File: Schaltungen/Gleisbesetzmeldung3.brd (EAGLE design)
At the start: 81 parts, among them IC1 CNY-17-2, IC10 S462, IC11 CNY-17-2, IC12 S462, IC13 CNY-17-2, IC14 S462, IC15 CNY-17-2, IC16 S462, IC2 S462, IC3 CNY-17-2, IC4 S462, IC5 CNY-17-2, IC6 S462, IC7 CNY-17-2, IC8 S462, IC9 CNY-17-2

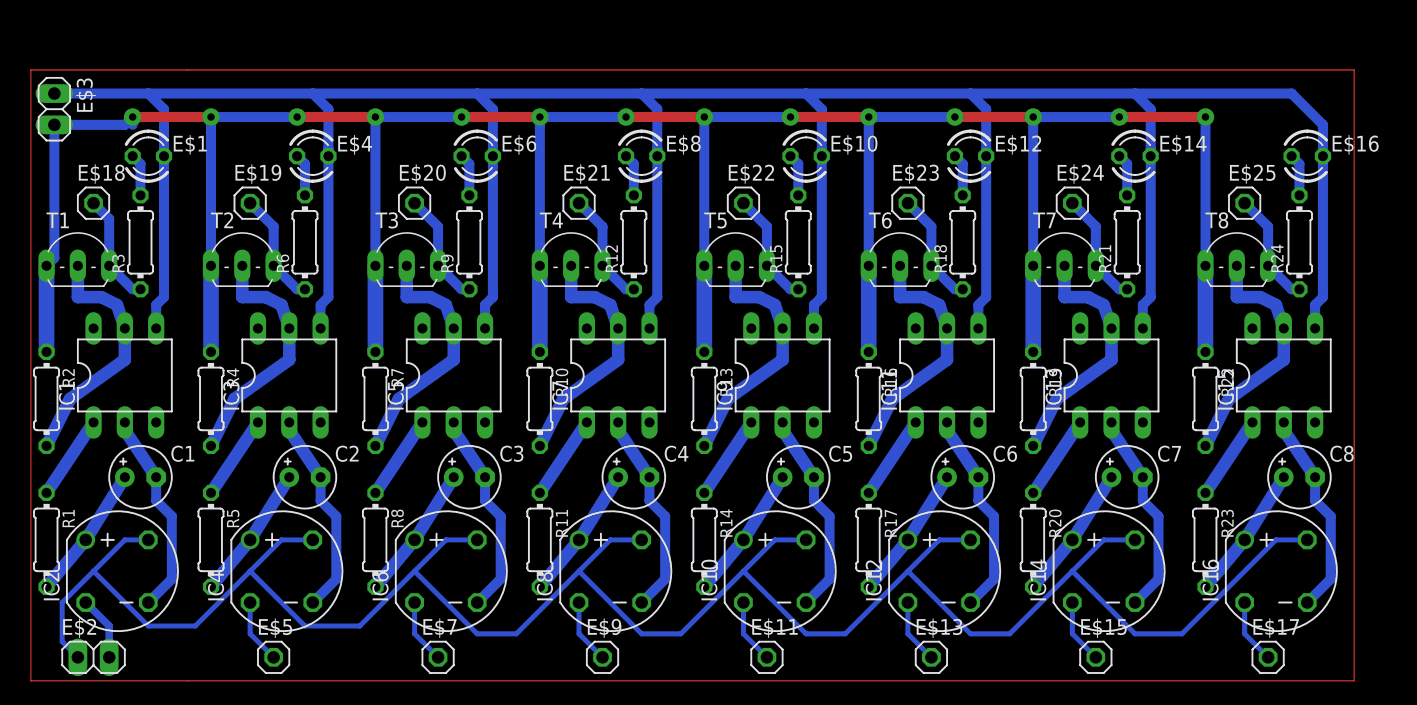
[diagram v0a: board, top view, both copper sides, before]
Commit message: update
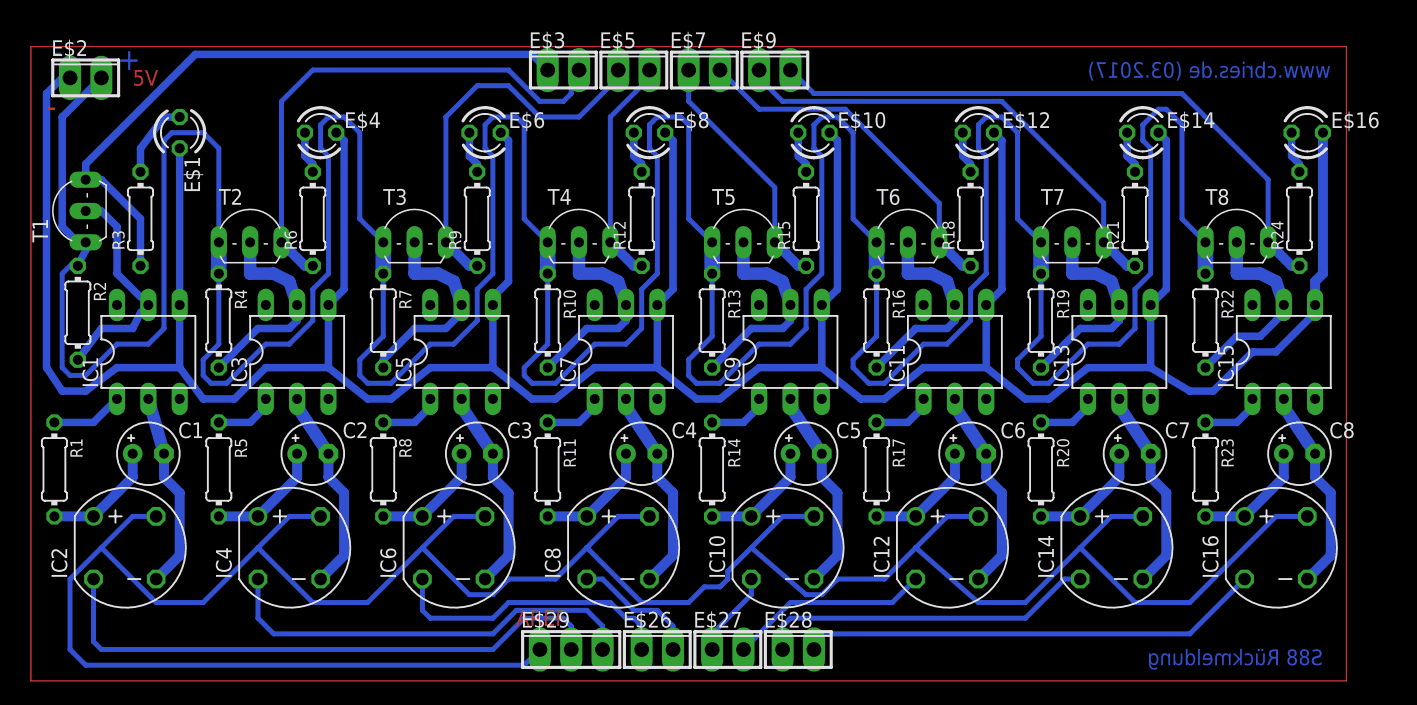
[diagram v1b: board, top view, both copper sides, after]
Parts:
- removed E$11, E$13, E$15, E$17, E$18, E$19, E$20, E$21, E$22, E$23, E$24, E$25: (no value), pinhead:1X01
- added E$26, E$27, E$28: (no value), con-phoenix-254:2POL254
- added E$29: (no value), con-phoenix-254:3POL254
- E$2, E$3: device pinhead:1X02 -> con-phoenix-254:2POL254
- E$5, E$7, E$9: device pinhead:1X01 -> con-phoenix-254:2POL254
- moved E$5 55.9 mm to (48.9, 49.5)
- moved E$7 52.3 mm to (54.6, 49.5)
- moved E$9 49.6 mm to (60.3, 49.5)
- moved E$2 47.0 mm to (4.45, 48.9)
- moved E$3 41.4 mm to (43.2, 49.5), turned to 0 degrees
- moved R2 7.43 mm to (3.81, 29.8)
- moved R16 6.38 mm to (68.6, 29.2)
- moved R19 6.38 mm to (81.9, 29.2)
- moved R10 6.38 mm to (41.9, 29.2)
- moved R13 6.38 mm to (55.2, 29.2)
- moved R4 6.38 mm to (15.2, 29.2)
- moved R7 6.38 mm to (28.6, 29.2)
- moved R22 6.35 mm to (95.2, 29.2)
- moved R17 5.75 mm to (68.6, 17.1)
- moved R20 5.75 mm to (81.9, 17.1)
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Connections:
- net S$130 renamed S$2
- removed net S$123: R4.1, T2.C
- removed net S$129: R7.1, T3.C
- removed net S$141: R13.1, T5.C
- removed net S$4: IC1.5, IC1.6, R2.2, T1.B
- net S$162: now also E$26.1, E$26.2, E$27.1, E$27.2, E$28.1, E$28.2, E$29.1, E$29.2, E$29.3; no longer E$11.1, E$13.1, E$15.1, E$17.1, E$2.1, E$2.2, E$5.1, E$7.1, E$9.1
- net S$3: now also E$2.2, IC1.5, IC1.6, R13.1, R2.2, R4.1, R7.1, T1.B, T2.C, T3.C, T5.C; no longer E$3.2
- net S$5: now also E$2.1, E$3.2, E$5.1, E$5.2, E$7.1, E$7.2, E$9.1, E$9.2; no longer E$18.1, E$19.1, E$20.1, E$21.1, E$22.1, E$23.1, E$24.1, E$25.1
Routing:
- net S$5: track 365.5 -> 605.7 mm
- net S$3: track 200.6 -> 409.2 mm, vias 14 -> 0
- net S$162: track 354.1 -> 552.3 mm
- net S$4: track 20.1 -> 0.00 mm
- net S$141: track 18.4 -> 0.00 mm
- net S$129: track 18.4 -> 0.00 mm
- net S$123: track 6.98 -> 0.00 mm
- net S$2: track 20.1 -> 16.4 mm
- net S$160: track 20.1 -> 16.7 mm
- net S$154: track 20.1 -> 17.1 mm
- net S$136: track 20.1 -> 17.1 mm
- net S$124: track 20.1 -> 17.1 mm
- net S$142: track 20.1 -> 17.1 mm
- net S$148: track 20.1 -> 17.1 mm
- net S$1: track 313.7 -> 316.2 mm
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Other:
- board text added: "+"
- board text added: "-"
- board text added: "5V"
- board text added: "AREF"
- board text added: "S88 Rückmeldung"
- board text added: "www.cbries.de (03.2017)"
